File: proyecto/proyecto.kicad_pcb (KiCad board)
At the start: 2 copper layers, 109 parts, among them J1 Conn_01x03, J2 Conn_01x03, J3 USB_A, J4 Conn_ARM_JTAG_SWD_20, J5 USB_B_Mini, J6 USB_A, J7 Conn_ARM_JTAG_SWD_20, J8 USB_B_Mini, J9 Conn_ARM_JTAG_SWD_20, Q1 Q_PMOS_DSG, Q2 Q_PMOS_DSG, SW1 SW_Push, SW2 SW_Push, SW3 SW_Push, U1 DRV8848, U10 STM32L052C6Tx, U11 LM1117-5.0, U12 LM1117-5.0, U2 Omega2+, U3 MCP73811T-435I-OT, U4 LM1117-3.3, U5 TPS61200DRC, U6 Omega2+, U7 LM1117-3.3, U8 MCP73811T-435I-OT, U9 TPS61200DRC, Y1 24M

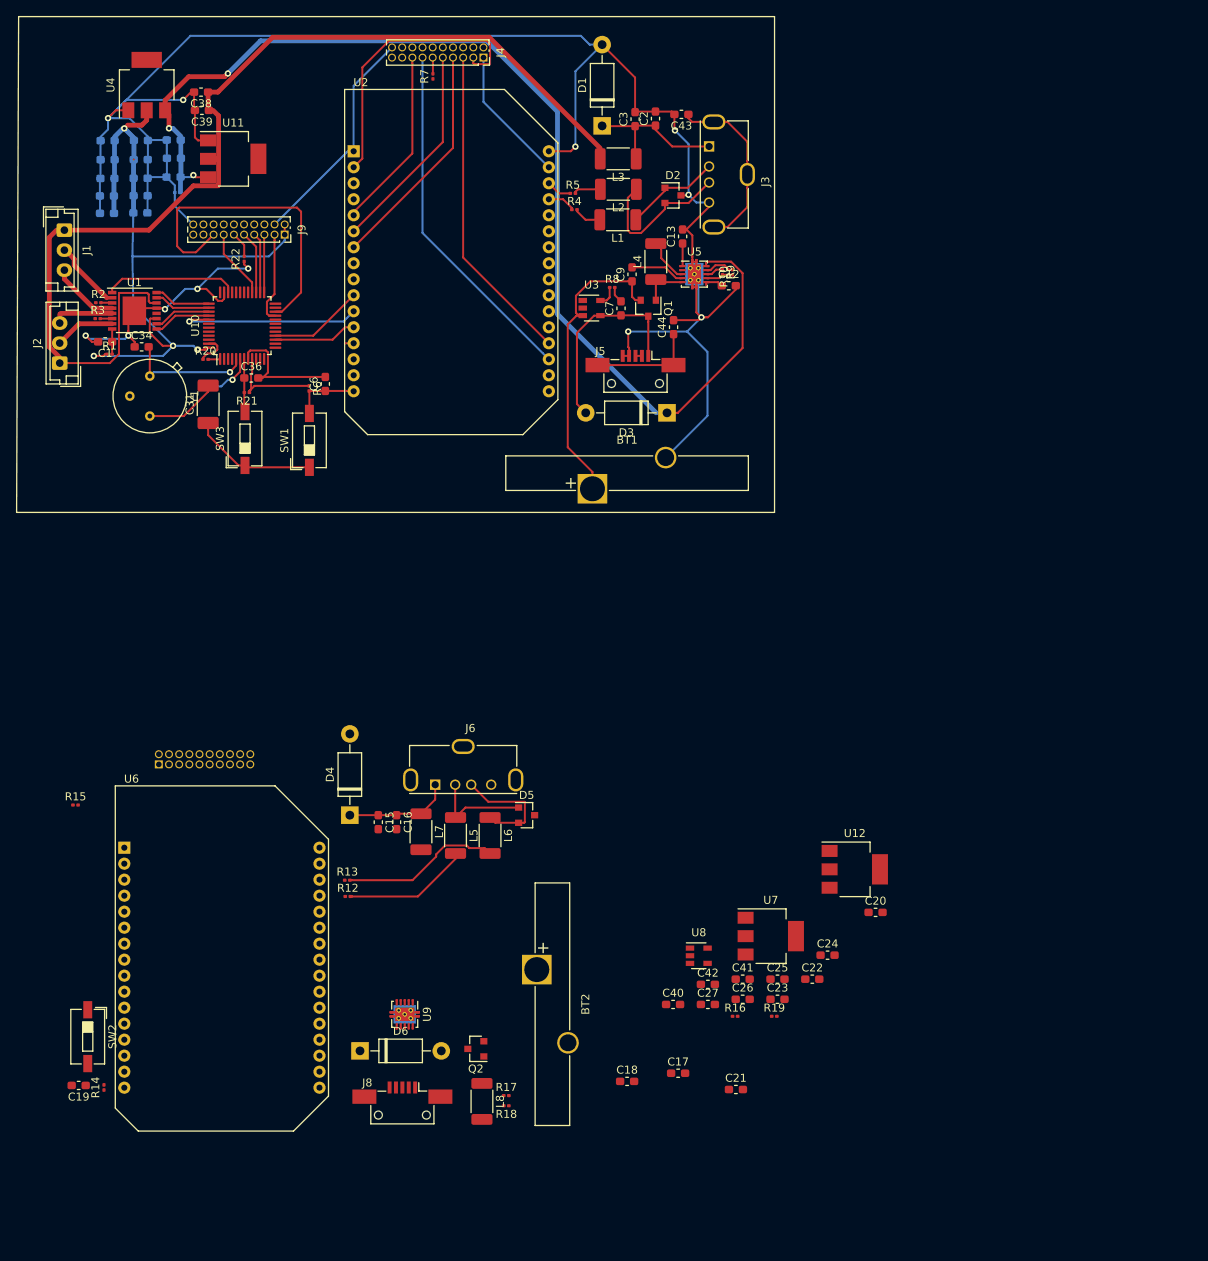
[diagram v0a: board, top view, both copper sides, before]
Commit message: Add files via upload
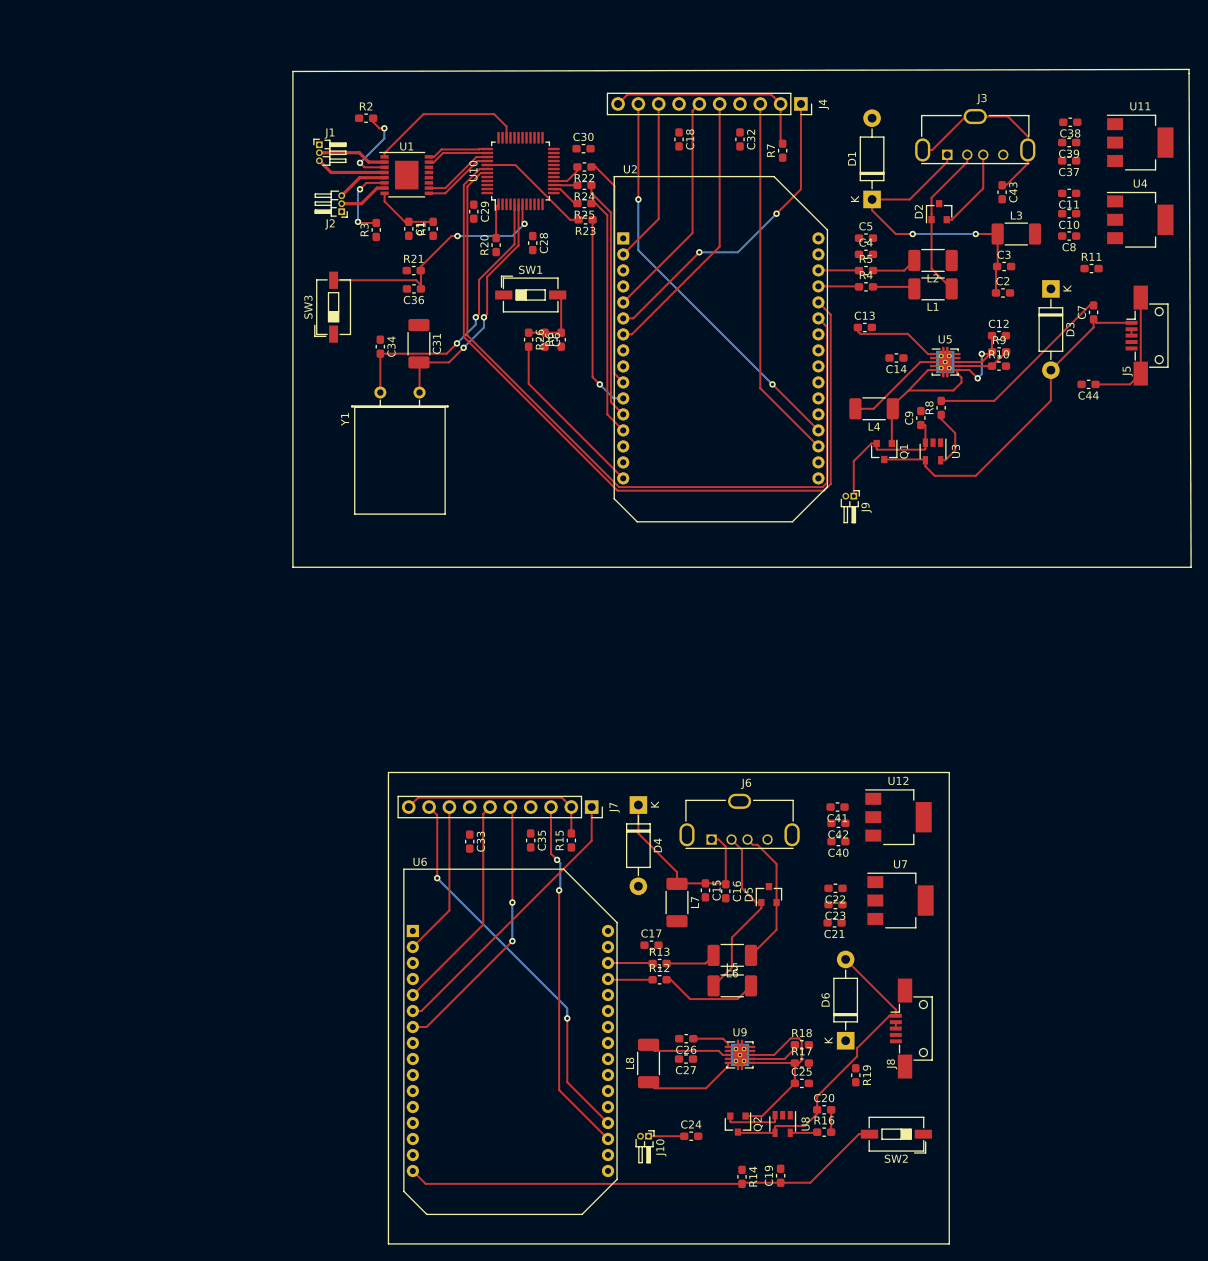
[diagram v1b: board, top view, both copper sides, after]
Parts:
- removed BT1: Battery_Cell_1, Battery:Battery_Panasonic_CR3032-VCN_Vertical_CircularHoles
- removed BT2: Battery_Cell_2, Battery:Battery_Panasonic_CR3032-VCN_Vertical_CircularHoles
- added J10: Conn_01x02, Connector_PinHeader_1.00mm:PinHeader_1x02_P1.00mm_Horizontal, F.Cu at (110.0, 163.3)
- added R23: 100, Resistor_SMD:R_0603_1608Metric_Pad1.05x0.95mm_HandSolder, F.Cu at (102.1, 48.8)
- added R24: 100, Resistor_SMD:R_0603_1608Metric_Pad1.05x0.95mm_HandSolder, F.Cu at (102.0, 44.5)
- added R25: 100, Resistor_SMD:R_0603_1608Metric_Pad1.05x0.95mm_HandSolder, F.Cu at (102.0, 46.7)
- added R26: 100, Resistor_SMD:R_0603_1608Metric_Pad1.05x0.95mm_HandSolder, F.Cu at (95.0, 63.8)
- C10, C11, C14, C28, C29, C30, C37, C4, C5, C8: moved to F.Cu
- C32, C33, C35: value 0.1uM -> 0.1uF; moved to F.Cu
- J1, J2: footprint Connector_JST:JST_EH_B3B-EH-A_1x03_P2.50mm_Vertical -> Connector_PinHeader_1.00mm:PinHeader_1x03_P1.00mm_Horizontal
- J4: value Conn_ARM_JTAG_SWD_20 -> AVR-JTAG-10; footprint Connector_PinSocket_1.27mm:PinSocket_2x10_P1.27mm_Vertical -> Connector_PinSocket_2.54mm:PinSocket_1x10_P2.54mm_Vertical
- J7: value Conn_ARM_JTAG_SWD_20 -> AVR-JTAG-10; footprint Connector_PinSocket_1.27mm:PinSocket_2x10_P1.27mm_Vertical -> Connector_PinSocket_2.54mm:PinSocket_1x10_P2.54mm_Vertical; moved to F.Cu
- J9: value Conn_ARM_JTAG_SWD_20 -> Conn_01x02; footprint Connector_PinSocket_1.27mm:PinSocket_2x10_P1.27mm_Vertical -> Connector_PinHeader_1.00mm:PinHeader_1x02_P1.00mm_Horizontal
- L1, L2, L3, L4, L5, L6, L7, L8: footprint Inductor_SMD:L_2010_5025Metric -> Inductor_SMD:L_2010_5025Metric_Pad1.52x2.65mm_HandSolder
- R1, R10, R12, R13, R14, R15, R16, R17, R18, R19, R2, R20, R21, R3, R4, R5, R6, R7, R8, R9: footprint Resistor_SMD:R_0201_0603Metric -> Resistor_SMD:R_0603_1608Metric_Pad1.05x0.95mm_HandSolder
- R11: footprint Resistor_SMD:R_0201_0603Metric -> Resistor_SMD:R_0603_1608Metric_Pad1.05x0.95mm_HandSolder; moved to F.Cu
- R22: value 510 -> 100; footprint Resistor_SMD:R_0201_0603Metric -> Resistor_SMD:R_0603_1608Metric_Pad1.05x0.95mm_HandSolder
- Y1: footprint Crystal:Crystal_HC35-U -> Crystal:Crystal_HC49-U_Horizontal
- moved U4 125.3 mm to (171.4, 48.8), turned to 0 degrees
- moved C18 117.9 mm to (113.8, 38.7), turned to 270 degrees
- moved C10 116.4 mm to (162.6, 48.0), turned to 180 degrees
- moved C11 116.1 mm to (162.6, 45.5), turned to 180 degrees
- moved R11 114.7 mm to (165.4, 54.9), turned to 0 degrees
- moved U11 113.4 mm to (171.4, 39.1)
- moved C8 112.3 mm to (162.6, 50.8)
- moved C37 112.0 mm to (162.6, 41.4)
- moved C38 108.7 mm to (162.7, 36.6)
- moved C39 108.5 mm to (162.6, 39.1)
- moved SW2 101.8 mm to (141.0, 163.1), turned to 180 degrees
- moved C35 96.1 mm to (95.2, 126.4), turned to 270 degrees
- moved C5 95.6 mm to (137.2, 51.1), turned to 0 degrees
- moved C14 94.4 mm to (141.0, 66.0)
- moved C4 90.9 mm to (137.2, 53.1)
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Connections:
- C18 pad 1: +3V0 -> +3V8
- C18 pad 2: GNDA -> GND
- C33 pad 1: +3V8 -> +3V0
- C33 pad 2: GND -> GNDA
- C35 pad 1: +3V8 -> +3V0
- C35 pad 2: GND -> GNDA
- C9 pad 1: Net-(BT1-Pad1) -> Net-(C9-Pad1)
- J4 pad 1: +3V8 -> /Procesador/TCK2
- J4 pad 10: GND -> Net-(J4-Pad10)
- J4 pad 2: +3V8 -> Net-(J4-Pad10)
- J4 pad 3: /Procesador/TRST2 -> /Procesador/TD02
- J4 pad 4: GND -> +3V8
- J4 pad 5: /Procesador/TD12 -> /Procesador/TMS2
- J4 pad 6: GND -> /Procesador/SRST2
- J4 pad 7: /Procesador/TMS2 -> +3V8
- J4 pad 8: GND -> /Procesador/TRST2
- J4 pad 9: /Procesador/TCK2 -> /Procesador/TD12
- J7 pad 1: +3V0 -> /camara/TCK3
- J7 pad 10: GNDA -> Net-(J7-Pad10)
- J7 pad 2: +3V0 -> Net-(J7-Pad10)
- J7 pad 3: /camara/TRST3 -> /camara/TD03
- J7 pad 4: GNDA -> +3V0
- J7 pad 5: /camara/TD13 -> /camara/TMS3
- J7 pad 6: GNDA -> /camara/SRST3
- J7 pad 7: /camara/TMS3 -> +3V0
- J7 pad 8: GNDA -> /camara/TRST3
- J7 pad 9: /camara/TCK3 -> /camara/TD13
- J9 pad 1: +3V8 -> Net-(C9-Pad1)
- J9 pad 2: +3V8 -> GND
- Q1 pad 2: Net-(BT1-Pad1) -> Net-(C9-Pad1)
- R15 pad 2: Net-(J7-Pad11) -> Net-(J7-Pad10)
- R22 pad 1: GND -> Net-(R22-Pad1)
- R22 pad 2: Net-(J9-Pad11) -> /Microcontrolador/MISO
- R7 pad 2: Net-(J4-Pad11) -> Net-(J4-Pad10)
- U10 pad 24: Net-(U10-Pad24) -> +3V8
- U2 pad 10: /Microcontrolador/MISO -> Net-(R22-Pad1)
- U2 pad 11: /Microcontrolador/MOSI -> Net-(R23-Pad1)
- U2 pad 12: /Microcontrolador/SCLK -> Net-(R24-Pad1)
- U2 pad 13: /Microcontrolador/CS1 -> Net-(R25-Pad1)
- U2 pad 16: /Procesador/RST_P -> Net-(R26-Pad2)
- U3 pad 3: Net-(BT1-Pad1) -> Net-(C9-Pad1)
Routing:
- net GND: track 353.2 -> 0.00 mm, vias 12 -> 0
- net +5VL: track 144.0 -> 0.00 mm, vias 3 -> 0
- net +5V: track 134.1 -> 0.00 mm
- net +3V8: track 119.7 -> 0.00 mm, vias 4 -> 0
- net /Microcontrolador/USART_1: track 0.00 -> 100.3 mm
- net /Microcontrolador/USART_2: track 0.00 -> 95.8 mm
- net /camara/RST_P2: track 0.00 -> 60.3 mm
- net /camara/TD13: track 0.00 -> 48.8 mm, vias 0 -> 2
- net /camara/TD03: track 0.00 -> 44.6 mm, vias 0 -> 2
- net /Microcontrolador/SRST1: track 40.5 -> 0.00 mm
- net Net-(C25-Pad1): track 0.00 -> 38.2 mm
- net Net-(BT1-Pad1): track 38.2 -> 0.00 mm
- net Net-(C20-Pad1): track 0.00 -> 37.8 mm
- net /camara/TCK3: track 0.00 -> 35.4 mm
- net /camara/TMS3: track 0.00 -> 33.8 mm, vias 0 -> 2
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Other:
- rule via_min_drill: 0.3 -> 0.4
- rule via_min_size: 0.4 -> 0.8
